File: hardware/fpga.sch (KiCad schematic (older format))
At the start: 0 parts

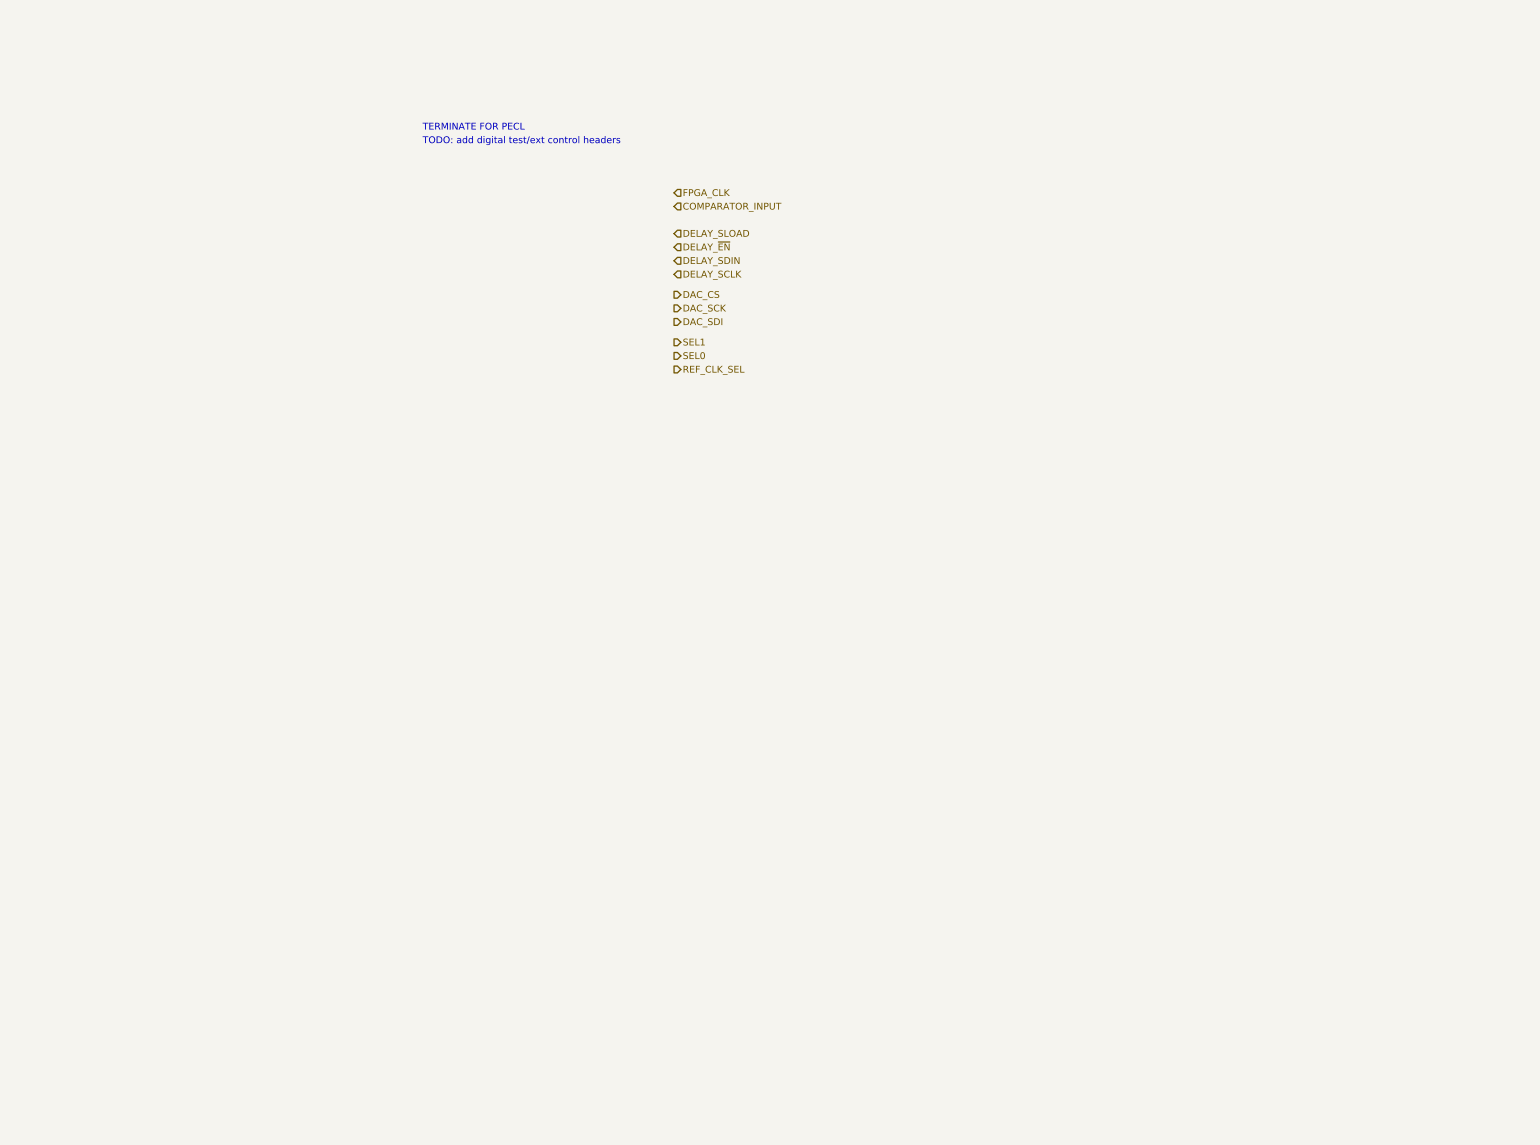
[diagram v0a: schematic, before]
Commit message: work on schematic..
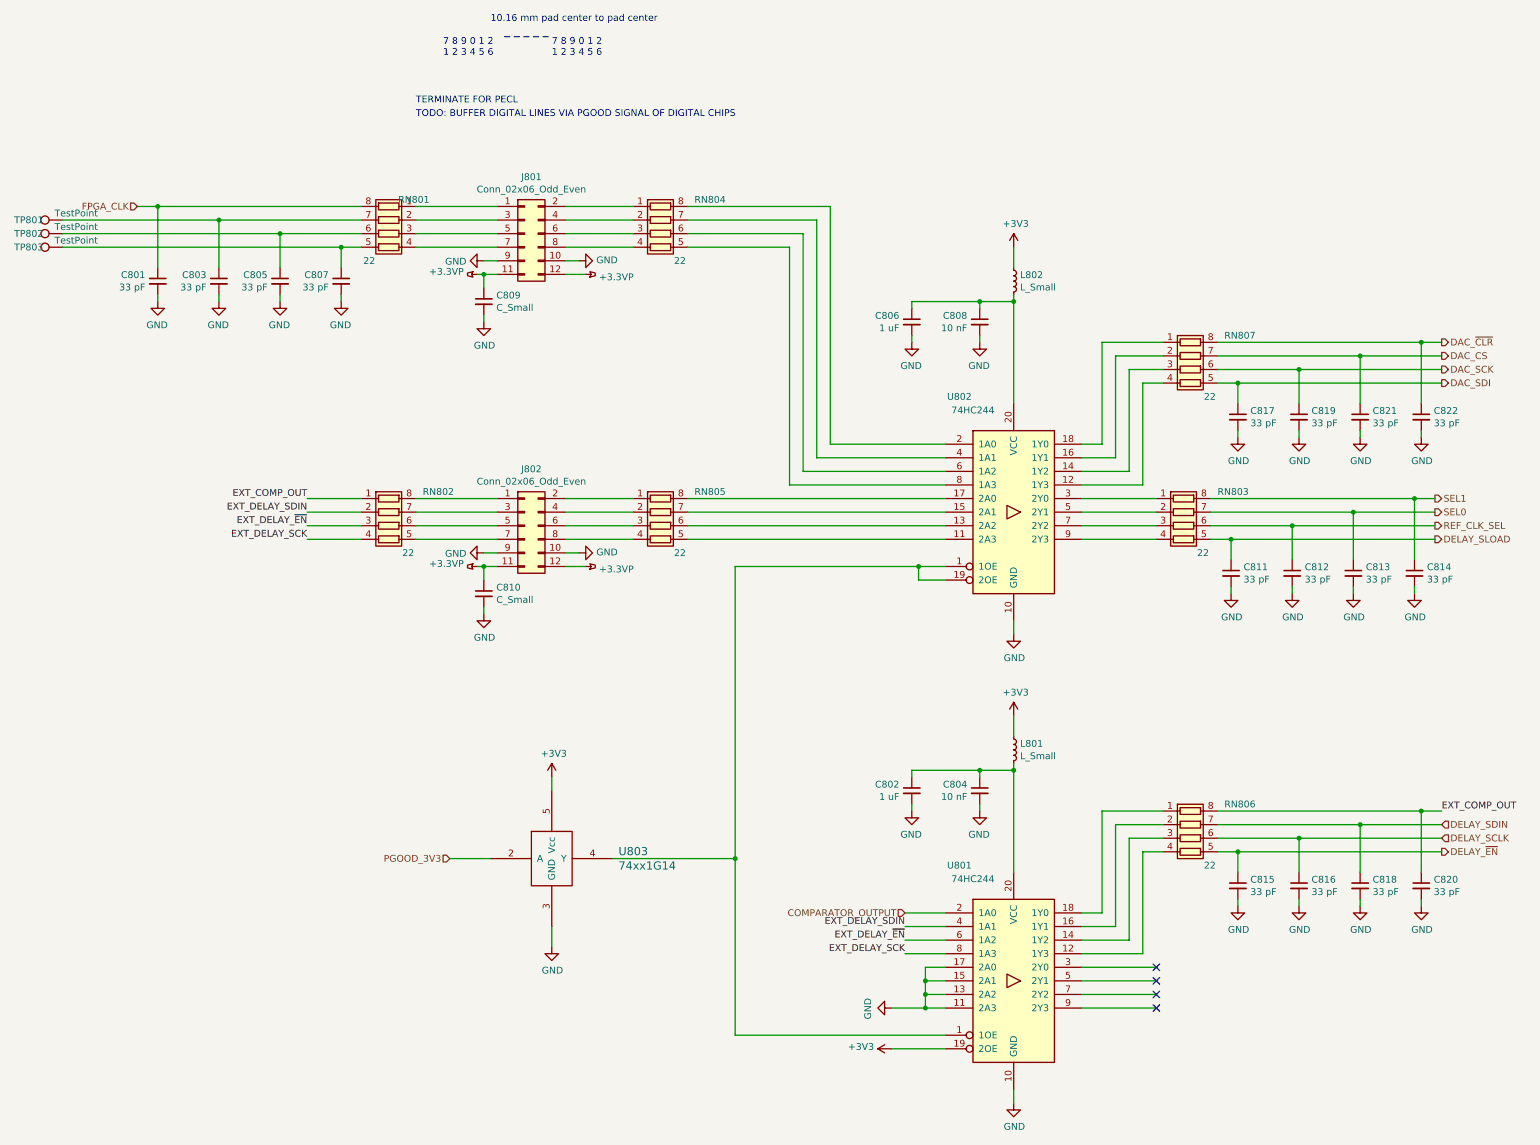
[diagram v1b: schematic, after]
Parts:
- added C801, C803, C805, C807, C811, C812, C813, C814, C815, C816, C817, C818, C819, C820, C821, C822: 33 pF, Capacitors_SMD:C_0402, symbol Device:C_Small
- added C802, C806: 1 uF, Capacitors_SMD:C_0603, symbol Device:C_Small
- added C804, C808: 10 nF, Capacitors_SMD:C_0402, symbol Device:C_Small
- added C809, C810: C_Small, Capacitors_SMD:C_0402, symbol Device:C_Small
- added J801, J802: Conn_02x06_Odd_Even, Pin_Headers:Pin_Header_Angled_2x06, symbol Connector_Generic:Conn_02x06_Odd_Even
- added L801, L802: L_Small, Resistors_SMD:R_0402, symbol Device:L_Small
- added RN801, RN802, RN803, RN804, RN805, RN806, RN807: 22, Resistors_SMD:R_Array_Convex_4x0402, symbol Device:R_Pack04
- added TP801, TP802, TP803: TestPoint, vna_footprints:TP07R, symbol Connector:TestPoint
- added U801, U802: 74HC244, Housings_SSOP:TSSOP-20_4.4x6.5mm_Pitch0.65mm, symbol 74xx:74HC244
- added U803: 74xx1G14, TO_SOT_Packages_SMD:SOT-23-5, symbol 74xx1g14:74xx1G14
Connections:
- net DAC_CS: now also C821.1, RN807.7 (R2.2)
- net DAC_SCK: now also C819.1, RN807.6 (R3.2)
- net DAC_SDI: now also C817.1, RN807.5 (R4.2)
- net DELAY_SCLK: now also C816.1, RN806.6 (R3.2)
- net DELAY_SDIN: now also C818.1, RN806.7 (R2.2)
- net DELAY_SLOAD: now also C811.1, RN803.5 (R4.2)
- net DELAY_~EN: now also C815.1, RN806.5 (R4.2)
- net FPGA_CLK: now also C801.1, RN801.8 (R1.2)
- net REF_CLK_SEL: now also C812.1, RN803.6 (R3.2)
- net SEL0: now also C813.1, RN803.7 (R2.2)
- net SEL1: now also C814.1, RN803.8 (R1.2)
- new net: U801.1 (1OE), U802.1 (1OE), U802.19 (2OE), U803.4 (Y)
- new net: RN805.5 (R4.2), U802.11 (2A3)
- new net: RN807.4 (R4.1), U802.12 (1Y3)
- new net: RN805.6 (R3.2), U802.13 (2A2)
- new net: RN807.3 (R3.1), U802.14 (1Y2)
- new net: RN805.7 (R2.2), U802.15 (2A1)
- new net: RN807.2 (R2.1), U802.16 (1Y1)
- new net: RN805.8 (R1.2), U802.17 (2A0)
- new net: RN807.1 (R1.1), U802.18 (1Y0)
- new net: RN804.8 (R1.2), U802.2 (1A0)
- new net: C806.1, C808.1, L802.2, U802.20 (VCC)
- new net: RN803.1 (R1.1), U802.3 (2Y0)
- new net: RN804.7 (R2.2), U802.4 (1A1)
- new net: RN803.2 (R2.1), U802.5 (2Y1)
- new net: RN804.6 (R3.2), U802.6 (1A2)
- new net: RN803.3 (R3.1), U802.7 (2Y2)
- new net: RN804.5 (R4.2), U802.8 (1A3)
- new net: RN803.4 (R4.1), U802.9 (2Y3)
- new net: J801.1 (Pin_1), RN801.1 (R1.1)
- new net: J801.3 (Pin_3), RN801.2 (R2.1)
- new net: J801.5 (Pin_5), RN801.3 (R3.1)
- new net: J801.7 (Pin_7), RN801.4 (R4.1)
- new net: C807.1, RN801.5 (R4.2), TP803.1
- new net: C805.1, RN801.6 (R3.2), TP802.1
- new net: C803.1, RN801.7 (R2.2), TP801.1
- new net: RN806.4 (R4.1), U801.12 (1Y3)
- new net: RN806.3 (R3.1), U801.14 (1Y2)
- new net: RN806.2 (R2.1), U801.16 (1Y1)
- new net: RN806.1 (R1.1), U801.18 (1Y0)
- new net: C802.1, C804.1, L801.2, U801.20 (VCC)
- new net: J802.7 (Pin_7), RN802.5 (R4.2)
- new net: J802.5 (Pin_5), RN802.6 (R3.2)
- new net: J802.3 (Pin_3), RN802.7 (R2.2)
- new net: J802.1 (Pin_1), RN802.8 (R1.2)
- new net: J801.2 (Pin_2), RN804.1 (R1.1)
- new net: J801.4 (Pin_4), RN804.2 (R2.1)
- new net: J801.6 (Pin_6), RN804.3 (R3.1)
- new net: J801.8 (Pin_8), RN804.4 (R4.1)
- new net: J802.2 (Pin_2), RN805.1 (R1.1)
- new net: J802.4 (Pin_4), RN805.2 (R2.1)
- new net: J802.6 (Pin_6), RN805.3 (R3.1)
- new net: J802.8 (Pin_8), RN805.4 (R4.1)
- new net +3.3VP: C809.1, C810.1, J801.11 (Pin_11), J801.12 (Pin_12), J802.11 (Pin_11), J802.12 (Pin_12)
- new net +3V3: L801.1, L802.1, U801.19 (2OE), U803.5 (Vcc)
- new net COMPARATOR_OUTPUT: U801.2 (1A0)
- new net DAC_~CLR: C822.1, RN807.8 (R1.2)
- new net EXT_COMP_OUT: C820.1, RN802.1 (R1.1), RN806.8 (R1.2)
- new net EXT_DELAY_SCK: RN802.4 (R4.1), U801.8 (1A3)
- new net EXT_DELAY_SDIN: RN802.2 (R2.1), U801.4 (1A1)
- new net EXT_DELAY_~EN: RN802.3 (R3.1), U801.6 (1A2)
- new net GND: C801.2, C802.2, C803.2, C804.2, C805.2, C806.2, C807.2, C808.2, C809.2, C810.2, C811.2, C812.2, C813.2, C814.2, C815.2, C816.2, C817.2, C818.2, C819.2, C820.2, C821.2, C822.2, J801.10 (Pin_10), J801.9 (Pin_9), J802.10 (Pin_10), J802.9 (Pin_9), U801.10 (GND), U801.11 (2A3), U801.13 (2A2), U801.15 (2A1), U801.17 (2A0), U802.10 (GND), U803.3 (GND)
- new net PGOOD_3V3: U803.2 (A)
- no-connect marks 0 -> 4
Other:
- note added: "10.16 mm pad center to pad center"
- note added: "7 8 9 0 1 2\n1 2 3 4 5 6"
- note added: "TODO: BUFFER DIGITAL LINES VIA PGOOD SIGNAL OF DIGITAL CHIPS"
- note removed: "TODO: add digital test/ext control headers"
